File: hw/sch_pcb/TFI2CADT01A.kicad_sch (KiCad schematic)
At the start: 38 parts, among them J1 SM04B-GHS-TB, J2 SM04B-GHS-TB, J3 SM04B-GHS-TB, J4 SM04B-GHS-TB, J5 SM04B-GHS-TB, J6 SM04B-GHS-TB, M1 HOLE, M2 HOLE, M3 HOLE, M4 HOLE, M5 HOLE, M6 HOLE, U1 MIC5504-3.3YM5, U2 LTC4317

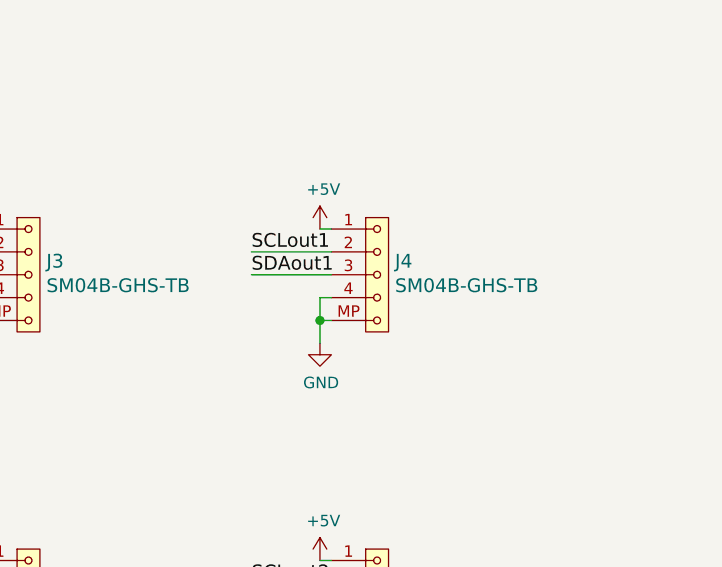
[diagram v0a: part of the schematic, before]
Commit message: uprava schema, sablona
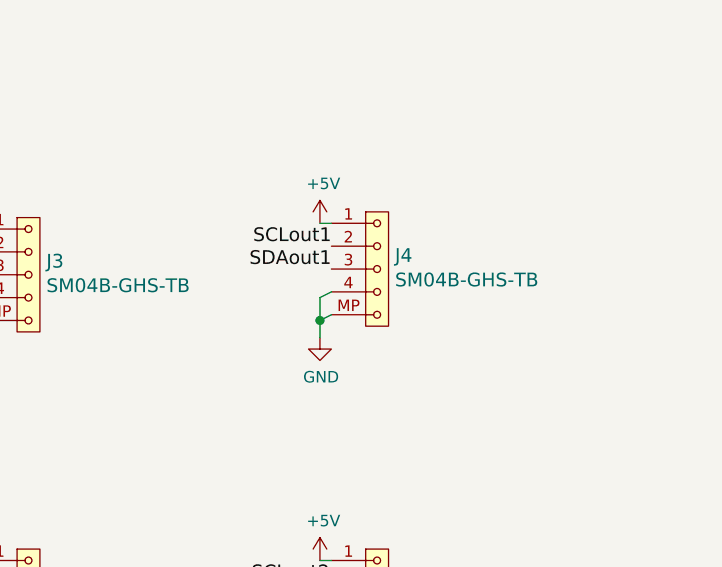
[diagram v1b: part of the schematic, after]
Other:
- moved on the sheet: J4
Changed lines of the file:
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@@
     (stroke (width 0) (type default) (color 0 0 0 0))
-  )
-  (wire (pts (xy 231.14 75.565) (xy 240.03 75.565))
-    (stroke (width 0) (type solid) (color 0 0 0 0))
   )
   (wire (pts (xy 40.64 165.1) (xy 40.64 166.37))
@@
     (stroke (width 0) (type solid) (color 0 0 0 0))
   )
-  (wire (pts (xy 240.03 80.645) (xy 238.76 80.645))
+  (wire (pts (xy 240.03 80.01) (xy 238.76 80.645))
     (stroke (width 0) (type solid) (color 0 0 0 0))
   )
@@
     (stroke (width 0) (type dash) (color 0 0 0 0))
   )
-  (wire (pts (xy 240.03 78.105) (xy 238.76 78.105))
+  (wire (pts (xy 240.03 77.47) (xy 238.76 78.105))
     (stroke (width 0) (type solid) (color 0 0 0 0))
   )
@@
     (stroke (width 0) (type default) (color 0 0 0 0))
   )
-  (wire (pts (xy 238.76 70.485) (xy 240.03 70.485))
-    (stroke (width 0) (type solid) (color 0 0 0 0))
-  )
-  (wire (pts (xy 238.76 80.645) (xy 238.76 83.185))
+  (wire (pts (xy 238.76 69.85) (xy 240.03 69.85))
+    (stroke (width 0) (type solid) (color 0 0 0 0))
+  )
+  (wire (pts (xy 238.76 80.645) (xy 238.76 82.55))
     (stroke (width 0) (type solid) (color 0 0 0 0))
   )
@@
   (wire (pts (xy 163.195 146.685) (xy 163.195 156.21))
     (stroke (width 0) (type default) (color 0 0 0 0))
-  )
-  (wire (pts (xy 231.14 73.025) (xy 240.03 73.025))
-    (stroke (width 0) (type solid) (color 0 0 0 0))
   )
   (wire (pts (xy 55.88 167.64) (xy 55.88 166.37))
@@
     (effects (font (size 1.524 1.524)) (justify left bottom))
   )
-  (label "SDAout1" (at 231.14 75.565 0) (fields_autoplaced)
-    (effects (font (size 1.524 1.524)) (justify left bottom))
+  (label "SDAout1" (at 240.03 74.93 180) (fields_autoplaced)
+    (effects (font (size 1.524 1.524)) (justify right bottom))
   )
   (label "SCLout1" (at 193.04 73.025 0) (fields_autoplaced)
@@
     (effects (font (size 1.524 1.524)) (justify right bottom))
   )
-  (label "SCLout1" (at 231.14 73.025 0) (fields_autoplaced)
-    (effects (font (size 1.524 1.524)) (justify left bottom))
+  (label "SCLout1" (at 240.03 72.39 180) (fields_autoplaced)
+    (effects (font (size 1.524 1.524)) (justify right bottom))
   )
   (label "SDAin" (at 77.47 83.185 180) (fields_autoplaced)
@@
     )
   )
-  (symbol (lib_id "power:GND") (at 238.76 83.185 0) (unit 1)
-    (in_bom yes) (on_board yes)
-    (property "Reference" "#PWR026" (id 0) (at 238.76 89.535 0)
-      (effects (font (size 1.27 1.27)) hide)
-    )
-    (property "Value" "GND" (id 1) (at 238.887 87.5792 0))
-    (property "Footprint" "" (id 2) (at 238.76 83.185 0)
-      (effects (font (size 1.27 1.27)) hide)
-    )
-    (property "Datasheet" "" (id 3) (at 238.76 83.185 0)
+  (symbol (lib_id "power:GND") (at 238.76 82.55 0) (unit 1)
+    (in_bom yes) (on_board yes)
+    (property "Reference" "#PWR026" (id 0) (at 238.76 88.9 0)
+      (effects (font (size 1.27 1.27)) hide)
+    )
+    (property "Value" "GND" (id 1) (at 238.887 86.9442 0))
+    (property "Footprint" "" (id 2) (at 238.76 82.55 0)
+      (effects (font (size 1.27 1.27)) hide)
+    )
+    (property "Datasheet" "" (id 3) (at 238.76 82.55 0)
       (effects (font (size 1.27 1.27)) hide)
     )
@@
     (pin "1")
   )
-  (symbol (lib_id "power:+5V") (at 238.76 70.485 0) (unit 1)
-    (in_bom yes) (on_board yes)
-    (property "Reference" "#PWR025" (id 0) (at 238.76 74.295 0)
-      (effects (font (size 1.27 1.27)) hide)
-    )
-    (property "Value" "+5V" (id 1) (at 239.141 66.0908 0))
-    (property "Footprint" "" (id 2) (at 238.76 70.485 0)
-      (effects (font (size 1.27 1.27)) hide)
-    )
-    (property "Datasheet" "" (id 3) (at 238.76 70.485 0)
-      (effects (font (size 1.27 1.27)) hide)
-    )
-    (pin "1")
-  )
-  (symbol (lib_id "MLAB_CONNECTORS_JST:SM04B-GHS-TB") (at 245.11 75.565 0) (unit 1)
-    (in_bom yes) (on_board yes)
-    (property "Reference" "J4" (id 0) (at 247.0912 74.0664 0)
+  (symbol (lib_id "power:+5V") (at 238.76 69.85 0) (unit 1)
+    (in_bom yes) (on_board yes)
+    (property "Reference" "#PWR025" (id 0) (at 238.76 73.66 0)
+      (effects (font (size 1.27 1.27)) hide)
+    )
+    (property "Value" "+5V" (id 1) (at 239.141 65.4558 0))
+    (property "Footprint" "" (id 2) (at 238.76 69.85 0)
+      (effects (font (size 1.27 1.27)) hide)
+    )
+    (property "Datasheet" "" (id 3) (at 238.76 69.85 0)
+      (effects (font (size 1.27 1.27)) hide)
+    )
+    (pin "1")
+  )
+  (symbol (lib_id "MLAB_CONNECTORS_JST:SM04B-GHS-TB") (at 245.11 74.93 0) (unit 1)
+    (in_bom yes) (on_board yes)
+    (property "Reference" "J4" (id 0) (at 247.0912 73.4314 0)
       (effects (font (size 1.524 1.524)) (justify left))
     )
-    (property "Value" "SM04B-GHS-TB" (id 1) (at 247.0912 76.7842 0)
+    (property "Value" "SM04B-GHS-TB" (id 1) (at 247.0912 76.1492 0)
       (effects (font (size 1.524 1.524)) (justify left))
     )
-    (property "Footprint" "Connector_JST:JST_GH_SM04B-GHS-TB_1x04-1MP_P1.25mm_Horizontal" (id 2) (at 245.11 70.485 0)
+    (property "Footprint" "Connector_JST:JST_GH_SM04B-GHS-TB_1x04-1MP_P1.25mm_Horizontal" (id 2) (at 245.11 69.85 0)
       (effects (font (size 1.524 1.524)) hide)
     )
-    (property "Datasheet" "" (id 3) (at 245.11 70.485 0)
-      (effects (font (size 1.524 1.524)))
-    )
-    (property "UST_id" "" (id 4) (at 245.11 75.565 0)
-      (effects (font (size 1.27 1.27)) hide)
-    )
-    (property "UST_ID" "5c86273d1287500b4e0280be" (id 5) (at 245.11 75.565 0)
-      (effects (font (size 1.27 1.27)) hide)
-    )
+    (property "Datasheet" "" (id 3) (at 245.11 69.85 0)
+      (effects (font (size 1.524 1.524)))
+    )
+    (property "UST_id" "" (id 4) (at 245.11 74.93 0)
+      (effects (font (size 1.27 1.27)) hide)
+    )
+    (property "UST_ID" "5c86273d1287500b4e0280be" (id 5) (at 245.11 74.93 0)
+      (effects (font (size 1.27 1.27)) hide)
+    )
